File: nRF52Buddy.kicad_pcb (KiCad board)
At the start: 4 copper layers, 60 x 35 mm, 98 parts, among them J1 2060-452_998-404, J2 SWD, J3 2305018-2, J4 Conn_02x26_Odd_Even, J5 Conn_02x26_Odd_Even, J6 S2B-PH-SM4-TB(LF)(SN), Q1 SSM3J332R, Q2 SSM3J332R, Q3 SSM3J332R, Q4 SSM3J332R, SW1 SW_SPST, U1 AP9211, U2 MAX17260SETD, U3 TP4054, U4 TP6841S6, U5 MIC5205-3.3YM5, U6 MDBT50Q-1MV2, U7 USBLC6-2SC6, Y1 32.768 kHz

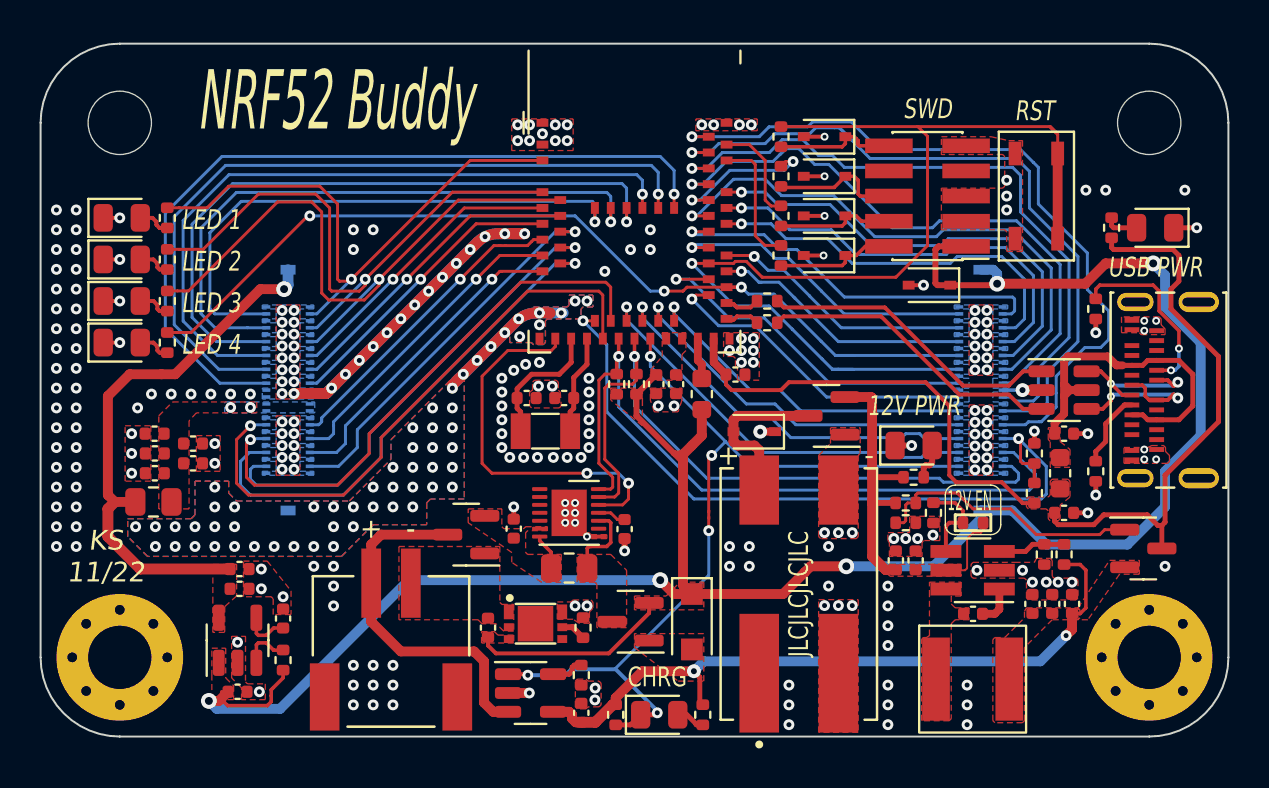
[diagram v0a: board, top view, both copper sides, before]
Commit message: Updates for revision 2
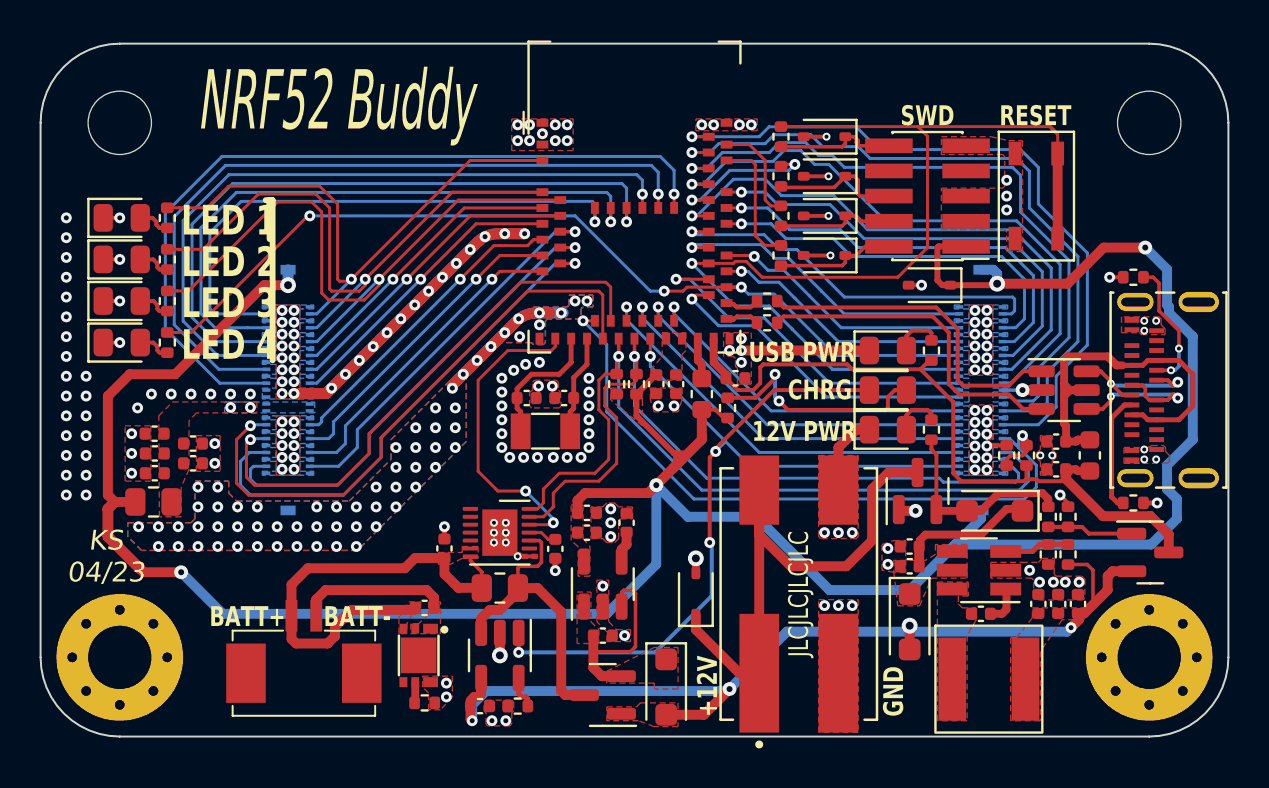
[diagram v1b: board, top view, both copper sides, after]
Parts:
- removed NT7: NetTie_2, Footprints:NetTie-2_SMD_Pad0.15mm
- removed Q4: SSM3J332R, Package_TO_SOT_SMD:SOT-23
- removed R23, R24, R25, R30: 10k, Resistor_SMD:R_0402_1005Metric
- added D14: D_Small, Diode_SMD:D_SOD-123F, F.Cu at (118.2, 115.8)
- added D15: D_Small, Diode_SMD:D_SOD-123F, F.Cu at (113.9, 121.4)
- J1: footprint SnapEDA Library:WAGO_2060-452_998-404 -> Footprints:WAGO_2060-452_998-404
- J3: footprint SnapEDA Library:TE_2305018-2 -> Footprints:TE_2305018-2
- J6: value S2B-PH-SM4-TB(LF)(SN) -> HDGC1251WR-S-2P; footprint Footprints:JST_S2B-PH-SM4-TB(LF)(SN) -> Footprints:HDGC1251WR-S-2P
- R32: value 10k -> 1k5
- R7: value 10 -> 10R
- SW1: footprint myFootprints:TS-1089S-02526 -> Footprints:TS-1089S-02526
- moved D16 20.1 mm to (112.8, 109.7)
- moved C14 18.7 mm to (98.4, 122.1)
- moved U5 18.7 mm to (98.4, 119.5)
- moved C13 18.0 mm to (99.6, 116.4)
- moved C11 17.8 mm to (97.6, 116.9)
- moved C12 17.8 mm to (97.6, 115.9)
- moved R32 15.6 mm to (104.7, 110.6), turned to -90 degrees
- moved D12 14.9 mm to (112.8, 107.7), turned to 0 degrees
- moved R21 11.0 mm to (115.0, 107.7)
- moved R1 8.86 mm to (89.4, 125.5), turned to 0 degrees
- moved D1 8.71 mm to (103.1, 120.0), turned to 90 degrees
- moved R5 8.21 mm to (121.9, 116.1), turned to -90 degrees
- moved R3 7.23 mm to (120.9, 116.1), turned to 90 degrees
- moved J6 6.33 mm to (83.3, 124.0), turned to 180 degrees
- moved U1 6.11 mm to (89.1, 123.1), turned to -90 degrees
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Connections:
- C19 pad 2: VCC -> +3V3
- C20 pad 2: VCC -> +3V3
- C3 pad 1: /Power Input/BATT_IN -> /Power Input/BATT_CONN+
- C4 pad 1: VCC -> /Power Input/BATT_CONN+
- C6 pad 1: /Power Input/+12V -> /Power Switching/12V_REG_IN
- C7 pad 1: /Power Input/+12V -> /Power Switching/12V_REG_IN
- D1 pad 1: GND -> /Power Input/+12V_CONN
- D1 pad 2: /Power Input/+12V_CONN -> GND
- D16 pad 1: /Power Input/~{CHARGE} -> /P1.09/~{CHARGE}
- D2 pad 1: VCC -> +3V3
- J2 pad 1: VCC -> +3V3
- J4 pad 48: /Connectors/P1.09 -> /P1.09/~{CHARGE}
- J4 pad 51: VCC -> +3V3
- J4 pad 52: VCC -> +3V3
- L3 pad 2: VCC -> +3V3
- R19 pad 2: VCC -> +3V3
- R2 pad 2: /Power Input/BATT_IN -> /Power Input/BATT_CONN+
- R20 pad 2: VCC -> +3V3
- R32 pad 2: +5V -> +3V3
- U1 pad 3: VCC -> /Power Input/BATT_CONN+
- U2 pad 6: /Power Input/BATT_IN -> /Power Input/BATT_CONN+
- U2 pad 7: /Power Input/BATT_IN -> /Power Input/BATT_CONN+
- U3 pad 1: /Power Input/~{CHARGE} -> /P1.09/~{CHARGE}
- U3 pad 3: /Power Input/BATT_CONN+ -> /Power Input/BATT+
- U4 pad 4: /Power Switching/12V EN -> /Power Switching/12V_REG_IN
- U4 pad 5: /Power Input/+12V -> /Power Switching/12V_REG_IN
- U5 pad 3: /Power Switching/3V3_EN -> VCC
- U6 pad 26: /Connectors/P1.09 -> /P1.09/~{CHARGE}
- U6 pad 28: VCC -> +3V3
- U6 pad 30: VCC -> +3V3
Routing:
- net +3V3: track 27.5 -> 137.5 mm, vias 1 -> 5
- net VCC: track 119.5 -> 9.57 mm, vias 5 -> 0
- net /P1.09/~{CHARGE}: track 0.00 -> 48.3 mm, vias 0 -> 4
- net /Connectors/P1.09: track 23.0 -> 0.00 mm, vias 2 -> 0
- net /Power Input/~{CHARGE}: track 20.6 -> 0.00 mm, vias 3 -> 0
- net /Power Input/+12V_CONN: track 8.44 -> 28.5 mm
- net /Power Switching/V_USB_FILT: track 50.6 -> 36.7 mm
- net +5V: track 35.3 -> 48.8 mm, vias 2 -> 4
- net /Power Input/BATT+: track 3.96 -> 15.2 mm
- net Net-(D16-A): track 1.57 -> 11.8 mm, vias 0 -> 2
- net GND: track 66.9 -> 76.7 mm, vias 318 -> 260
- net /Power Switching/12V__GATE_EN: track 13.9 -> 5.15 mm
- net /Power Input/+12V: track 18.5 -> 10.1 mm
- net /Power Input/BATT_CONN-: track 0.00 -> 7.65 mm
- net /Power Switching/12V_REG_IN: track 0.00 -> 7.29 mm
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- added copper zone on F.Cu, net /Power Input/BATT_CONN+
- added copper zone on F.Cu, net /Power Switching/12V_REG_IN
- removed copper zone on F.Cu, net /Power Input/+12V
- removed copper zone on F.Cu, net /Power Input/BATT+
- removed copper zone on F.Cu, net /Power Input/BATT_IN
- removed copper zone on F.Cu, net /Power Switching/V_USB
- removed copper zone on F.Cu, net /Power Switching/V_USB_FILT
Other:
- board text added: "+12V"
- board text added: "BATT+"
- board text added: "BATT-"
- board text added: "GND"
- board text added: "KS 04/23"
- board text added: "RESET"
- board text removed: "+"
- board text removed: "-"
- board text removed: "12V EN"
- board text removed: "KS 11/22"
- board text removed: "RST"

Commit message: updating bom
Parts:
- D1: value D_TVS -> D_TVS_15V
- D2, D3, D4, D5, D6: value D_TVS -> D_TVS_5V
